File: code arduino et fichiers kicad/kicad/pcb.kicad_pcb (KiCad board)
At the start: 2 copper layers, 53.5 x 80 mm, 46 parts, among them J1 Screw_Terminal_01x04, J2 Screw_Terminal_01x03, U1 LMC6482, U2 LMC6482, U3 LMC6482, U4 LMC6482

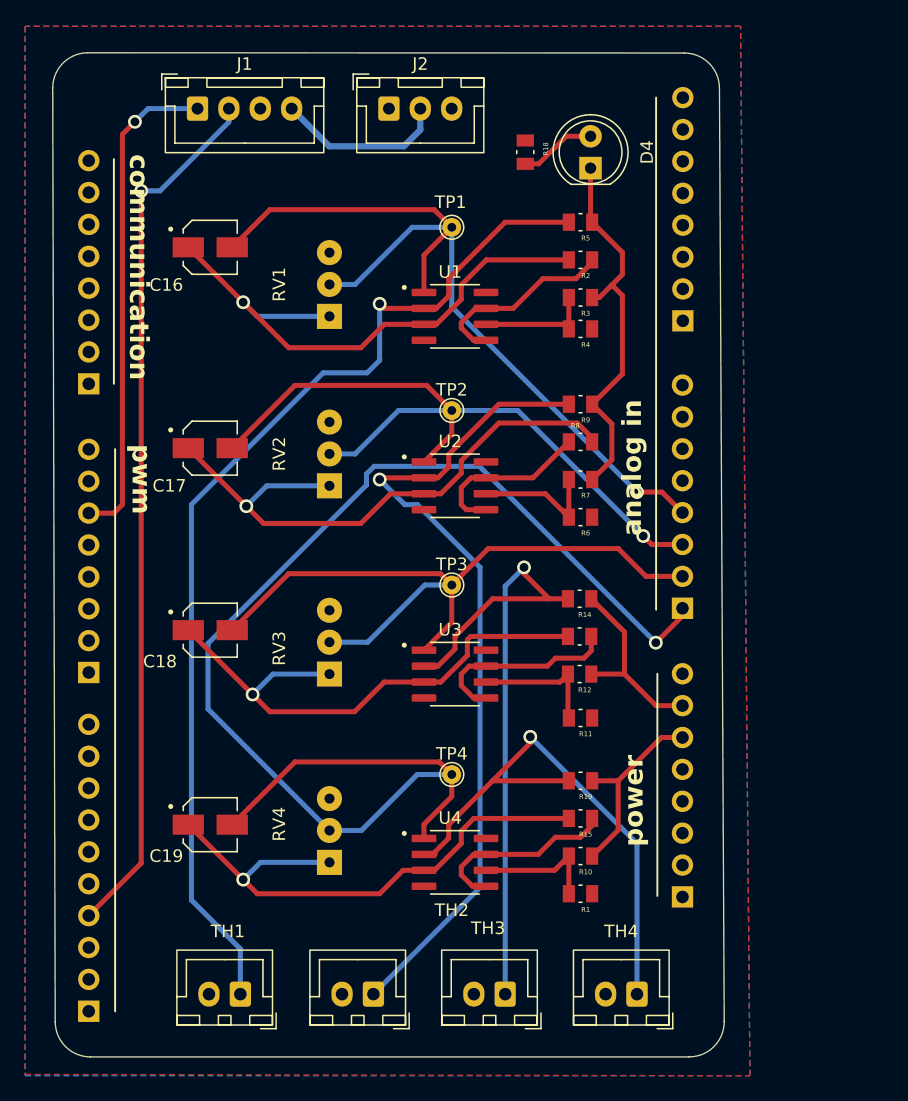
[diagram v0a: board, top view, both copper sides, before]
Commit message: PCB V2
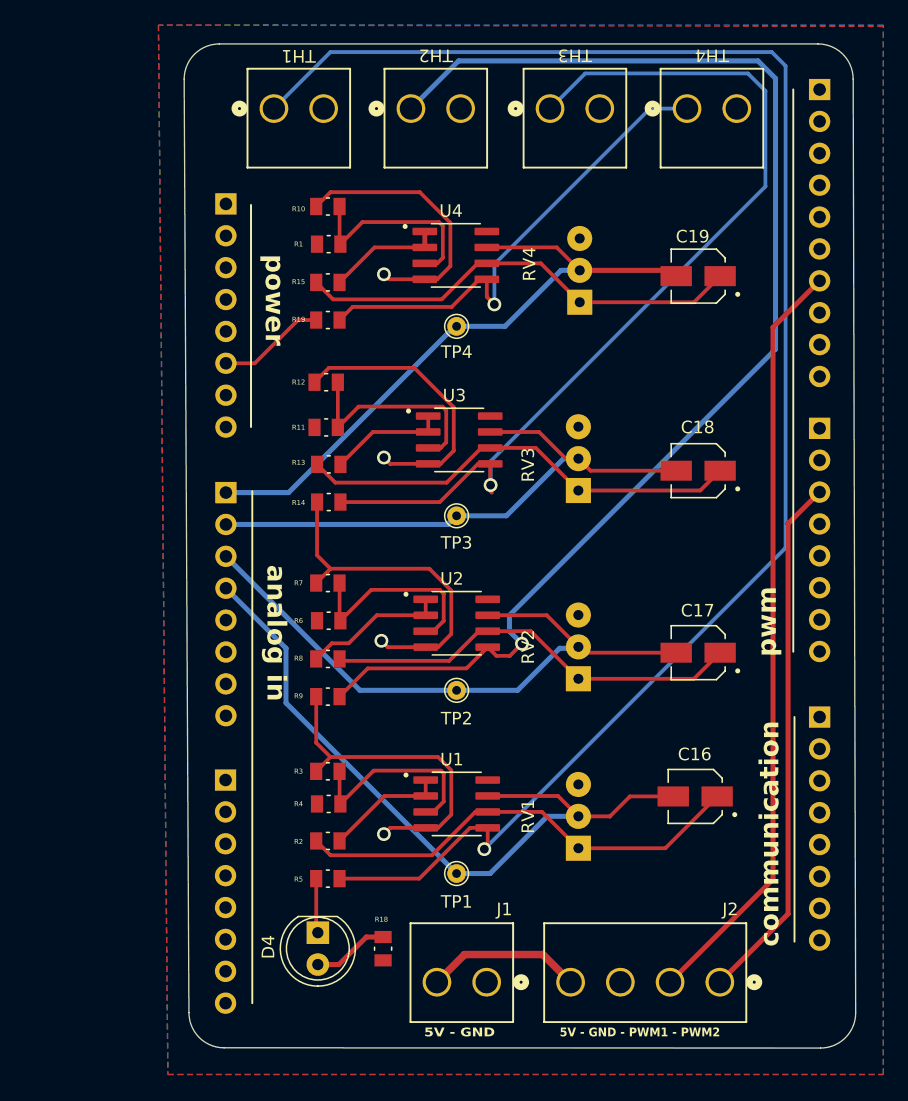
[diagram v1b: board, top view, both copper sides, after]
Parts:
- J1: value Screw_Terminal_01x04 -> MTA_02; footprint Connector_JST:JST_XH_B4B-XH-A_1x04_P2.50mm_Vertical -> ampli op:MTA_CONN2_640445-2
- J2: value Screw_Terminal_01x03 -> MTA_04; footprint Connector_JST:JST_XH_B3B-XH-A_1x03_P2.50mm_Vertical -> ampli op:MTA_CONN4_640445-4
- TH1, TH2, TH3, TH4: footprint Connector_JST:JST_XH_B2B-XH-A_1x02_P2.50mm_Vertical -> ampli op:MTA_CONN2_640445-2
- U1, U2, U3, U4: value LMC6482 -> LMC6482IMX_NOPB
- moved pwm1 93.7 mm to (131.9, 47.7), turned to 180 degrees
- moved J2 74.4 mm to (124.0, 118.8)
- moved J1 73.3 mm to (105.4, 118.8)
- moved TH4 70.7 mm to (121.4, 49.2)
- moved TH3 70.6 mm to (110.4, 49.2)
- moved TH2 70.6 mm to (99.4, 49.2)
- moved TH1 70.6 mm to (88.4, 49.2)
- moved power2 66.1 mm to (84.6, 56.8), turned to 180 degrees
- moved D4 64.7 mm to (91.9, 114.9), turned to -90 degrees
- moved R18 64.5 mm to (97.1, 116.1), turned to 90 degrees
- moved comm1 64.0 mm to (131.9, 97.7), turned to 180 degrees
- moved pwm2 61.4 mm to (131.9, 74.7), turned to 180 degrees
- moved C19 58.5 mm to (122.2, 62.5), turned to 180 degrees
- moved C16 58.4 mm to (122.0, 104.0), turned to 180 degrees
- moved R5 56.0 mm to (92.7, 110.5), turned to 0 degrees
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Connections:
- C16 pad 1: Net-(U1A-+) -> Net-(U1-NEGB)
- C17 pad 1: Net-(U2A-+) -> Net-(U2-NEGB)
- C18 pad 1: Net-(U3A-+) -> Net-(U3-NEGB)
- C19 pad 1: Net-(U4A-+) -> Net-(U4-NEGB)
- J1 pad 1: pwmdroite -> GND
- J1 pad 2: pwmgauche -> +5V (Ali seulement)
- J2 pad 1: GND -> pwmdroite
- J2 pad 2: +5V (Ali seulement) -> pwmgauche
- J2 pad 3: unconnected-(J2-Pin_3-Pad3) -> GND
- R1 pad 1: +5V -> Net-(U4-POSA)
- R1 pad 2: Net-(U4B--) -> +5V
- R10 pad 1: GND -> Net-(U4-POSA)
- R10 pad 2: Net-(U4B--) -> GND
- R11 pad 2: Net-(U3B--) -> Net-(U3-POSA)
- R12 pad 2: Net-(U3B--) -> Net-(U3-POSA)
- R13 pad 1: Net-(U3B-+) -> Net-(U3-NEGB)
- R13 pad 2: Net-(U3A-+) -> Net-(U3-NEGA)
- R14 pad 1: GND -> Net-(U3-POSB)
- R14 pad 2: Net-(U3A--) -> GND
- R15 pad 1: Net-(U4B-+) -> Net-(U4-NEGB)
- R15 pad 2: Net-(U4A-+) -> Net-(U4-NEGA)
- R19 pad 1: GND -> Net-(U4-POSB)
- R19 pad 2: Net-(U4A--) -> GND
- R2 pad 1: Net-(U1B-+) -> Net-(U1-NEGB)
- R2 pad 2: Net-(U1A-+) -> Net-(U1-NEGA)
- R3 pad 2: Net-(U1B--) -> Net-(U1-POSA)
- R4 pad 2: Net-(U1B--) -> Net-(U1-POSA)
- R5 pad 2: Net-(U1A--) -> Net-(U1-POSB)
- R6 pad 2: Net-(U2B--) -> Net-(U2-POSA)
- R7 pad 2: Net-(U2B--) -> Net-(U2-POSA)
- R8 pad 1: Net-(U2B-+) -> Net-(U2-NEGB)
- R8 pad 2: Net-(U2A-+) -> Net-(U2-NEGA)
- R9 pad 1: GND -> Net-(U2-POSB)
- R9 pad 2: Net-(U2A--) -> GND
- RV1 pad 1: Net-(U1A-+) -> Net-(U1-NEGB)
- RV2 pad 1: Net-(U2A-+) -> Net-(U2-NEGB)
- RV3 pad 1: Net-(U3A-+) -> Net-(U3-NEGB)
- RV4 pad 1: Net-(U4A-+) -> Net-(U4-NEGB)
- TH1 pad 1: Net-(U1A--) -> Net-(U1-POSB)
- TH2 pad 1: Net-(U2A--) -> Net-(U2-POSB)
- TH3 pad 1: Net-(U3A--) -> Net-(U3-POSB)
- TH4 pad 1: Net-(U4A--) -> Net-(U4-POSB)
- U1 pad 1: T1 sortie -> Net-(U1-NEGA)
- U1 pad 2: Net-(U1A--) -> Net-(U1-NEGA)
- U1 pad 3: Net-(U1A-+) -> Net-(U1-POSA)
- U1 pad 4: (no net) -> GND
- U1 pad 5: Net-(U1B-+) -> Net-(U1-POSB)
- U1 pad 6: Net-(U1B--) -> Net-(U1-NEGB)
- U1 pad 7: Net-(U1B-+) -> T1 sortie
- U1 pad 8: (no net) -> +5V
- U2 pad 1: T2 sortie -> Net-(U2-NEGA)
- U2 pad 2: Net-(U2A--) -> Net-(U2-NEGA)
- U2 pad 3: Net-(U2A-+) -> Net-(U2-POSA)
- U2 pad 4: (no net) -> GND
- U2 pad 5: Net-(U2B-+) -> Net-(U2-POSB)
- U2 pad 6: Net-(U2B--) -> Net-(U2-NEGB)
- U2 pad 7: Net-(U2B-+) -> T2 sortie
- U2 pad 8: (no net) -> +5V
- U3 pad 1: T3 sortie -> Net-(U3-NEGA)
- U3 pad 2: Net-(U3A--) -> Net-(U3-NEGA)
- U3 pad 3: Net-(U3A-+) -> Net-(U3-POSA)
- U3 pad 4: (no net) -> GND
- U3 pad 5: Net-(U3B-+) -> Net-(U3-POSB)
- U3 pad 6: Net-(U3B--) -> Net-(U3-NEGB)
- U3 pad 7: Net-(U3B-+) -> T3 sortie
- U3 pad 8: (no net) -> +5V
- U4 pad 1: T4 sortie -> Net-(U4-NEGA)
- U4 pad 2: Net-(U4A--) -> Net-(U4-NEGA)
- U4 pad 3: Net-(U4A-+) -> Net-(U4-POSA)
- U4 pad 4: (no net) -> GND
- U4 pad 5: Net-(U4B-+) -> Net-(U4-POSB)
- U4 pad 6: Net-(U4B--) -> Net-(U4-NEGB)
- U4 pad 7: Net-(U4B-+) -> T4 sortie
- U4 pad 8: (no net) -> +5V
- pwm1 pad 1: /D8 -> /SCL
- pwm1 pad 10: /SCL -> /D8
- pwm1 pad 2: /D9 -> /SDA
- pwm1 pad 3: /D10 -> +AREF
- pwm1 pad 4: pwmgauche -> GND
- pwm1 pad 5: /D12 -> /D13
- pwm1 pad 6: /D13 -> /D12
- pwm1 pad 7: GND -> pwmgauche
- pwm1 pad 8: +AREF -> /D10
- pwm1 pad 9: /SDA -> /D9
- pwm2 pad 1: /D0/RX0 -> /D7
- pwm2 pad 2: /D1/TX0 -> /D6
- pwm2 pad 3: /D2 -> pwmdroite
- pwm2 pad 4: /D3 -> /D4
- pwm2 pad 5: /D4 -> /D3
- pwm2 pad 6: pwmdroite -> /D2
- pwm2 pad 7: /D6 -> /D1/TX0
- pwm2 pad 8: /D7 -> /D0/RX0
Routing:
- net Net-(U1-POSB): track 0.00 -> 130.7 mm, vias 0 -> 1
- net Net-(U2-POSB): track 0.00 -> 102.3 mm, vias 0 -> 1
- net Net-(U1A--): track 83.8 -> 0.00 mm, vias 1 -> 0
- net Net-(U3-POSB): track 0.00 -> 74.9 mm, vias 0 -> 1
- net Net-(U2A--): track 66.6 -> 0.00 mm, vias 1 -> 0
- net T4 sortie: track 108.0 -> 51.6 mm, vias 1 -> 0
- net Net-(U3A--): track 52.2 -> 0.00 mm, vias 1 -> 0
- net GND: track 61.7 -> 110.9 mm, vias 0 -> 4
- net Net-(U2A-+): track 46.7 -> 0.00 mm, vias 1 -> 0
- net Net-(U1A-+): track 44.5 -> 0.00 mm, vias 1 -> 0
- net Net-(U4A--): track 44.3 -> 0.00 mm, vias 1 -> 0
- net Net-(U4A-+): track 43.1 -> 0.00 mm, vias 1 -> 0
- net Net-(U3A-+): track 43.0 -> 0.00 mm, vias 1 -> 0
- net Net-(U4-POSB): track 0.00 -> 39.0 mm, vias 0 -> 1
- net Net-(U1-NEGB): track 0.00 -> 36.8 mm
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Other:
- outline, holes or cut-outs redrawn
- board text added: "5V - GND"
- board text added: "5V - GND - PWM1 - PWM2"
- board text added: "R13"
- board text removed: "TH3"
